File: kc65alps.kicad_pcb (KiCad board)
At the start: 2 copper layers, 304.8 x 95.3 mm, 160 parts, among them J1 Conn_01x04, J2 AVR-ISP-6, U1 ATmega32U4-AU, Y1 16MHz

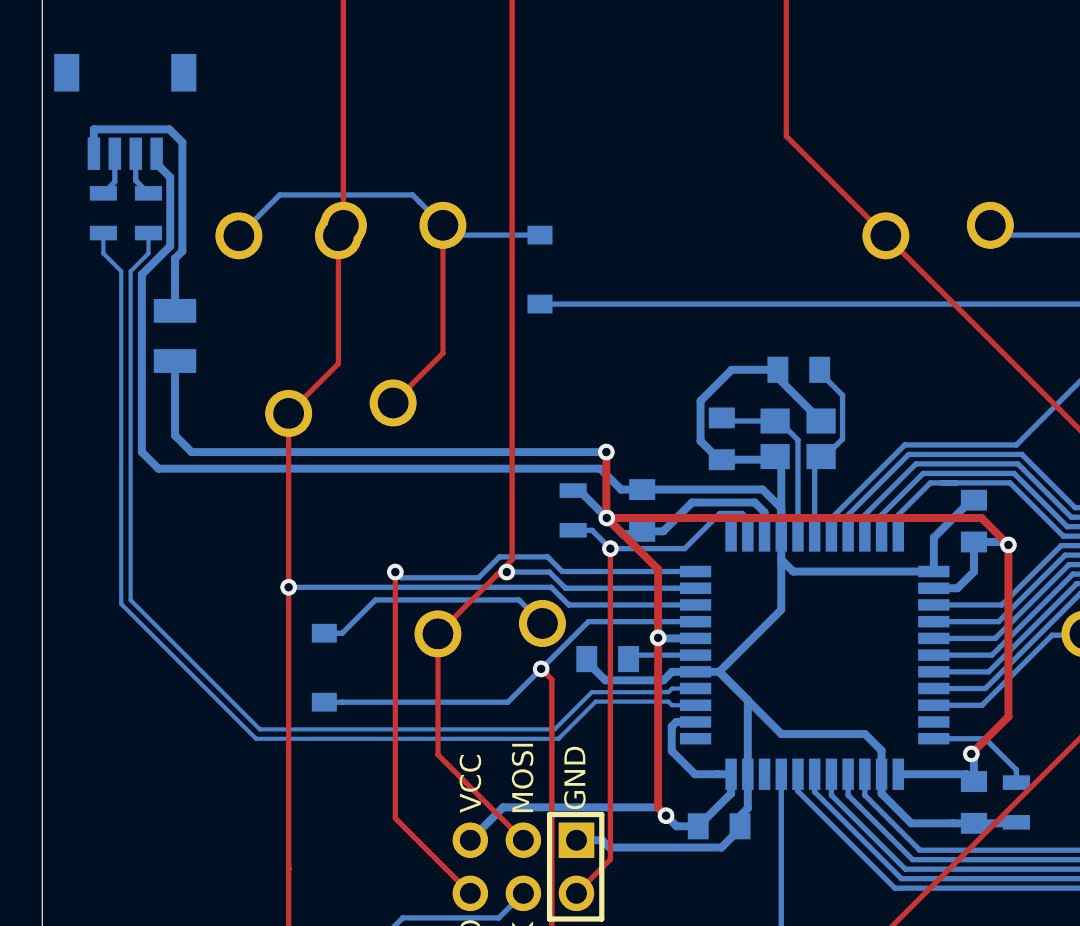
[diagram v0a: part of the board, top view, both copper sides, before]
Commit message: PCB update
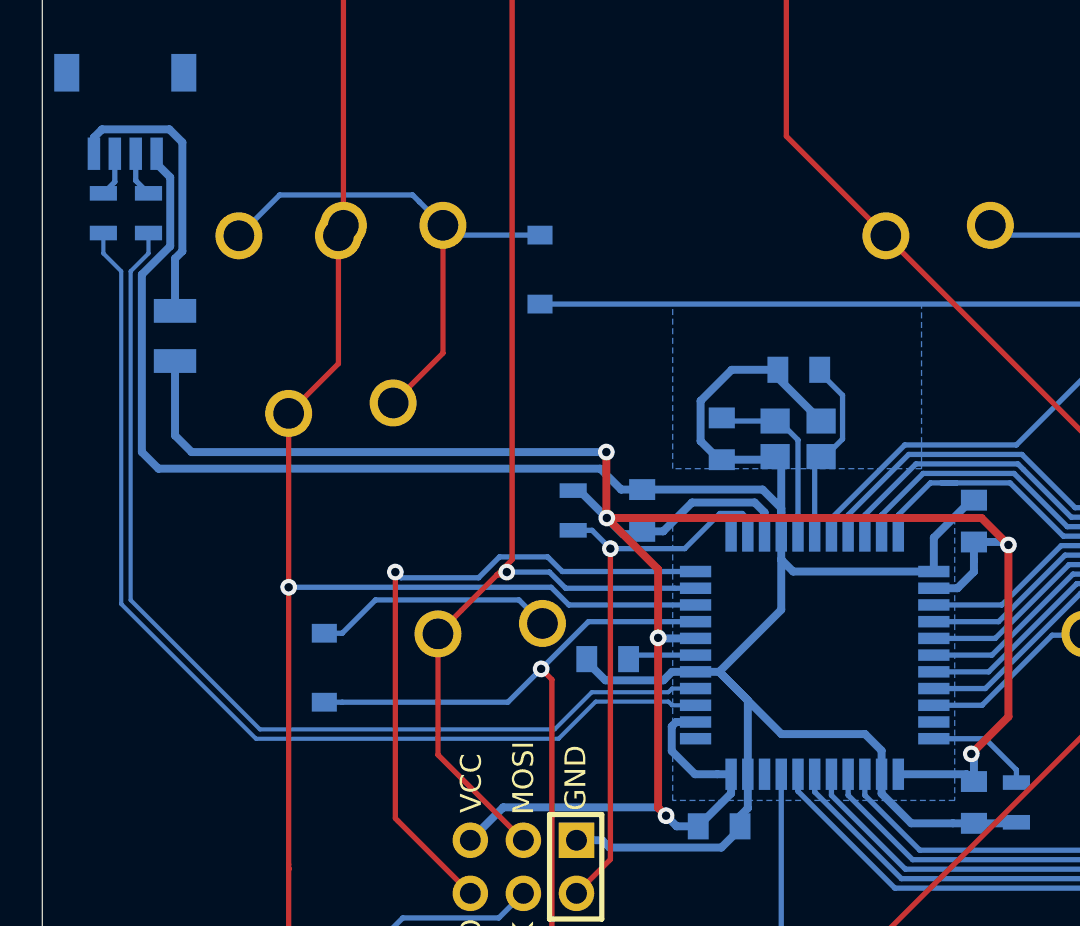
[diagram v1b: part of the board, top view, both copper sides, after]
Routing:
- added copper zone on B.Cu, net GND
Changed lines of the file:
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@@
   (segment (start 21.51875 119.075) (end 21.51875 119.55) (width 0.381) (layer B.Cu) (net 79))
   (segment (start 25.4 124.090357) (end 25.4 126.59375) (width 0.381) (layer B.Cu) (net 79))
-  (segment (start 21.51875 117.919) (end 21.528251 117.909499) (width 0.381) (layer B.Cu) (net 79))
-  (segment (start 21.51875 119.075) (end 21.51875 117.919) (width 0.381) (layer B.Cu) (net 79))
-  (segment (start 21.528251 117.909499) (end 25.131151 117.909499) (width 0.381) (layer B.Cu) (net 79))
+  (segment (start 21.51875 119.075) (end 21.51875 118.297098) (width 0.381) (layer B.Cu) (net 79))
+  (segment (start 21.906349 117.909499) (end 25.131151 117.909499) (width 0.381) (layer B.Cu) (net 79))
+  (segment (start 21.51875 118.297098) (end 21.906349 117.909499) (width 0.381) (layer B.Cu) (net 79))
   (segment (start 25.131151 117.909499) (end 25.751511 118.529859) (width 0.381) (layer B.Cu) (net 79))
   (segment (start 25.751511 118.529859) (end 25.751511 123.738846) (width 0.381) (layer B.Cu) (net 79))
@@
   (segment (start 64.1645 147.0655) (end 65.659 148.56) (width 0.254) (layer B.Cu) (net 100))
   (segment (start 61.707 147.0655) (end 64.1645 147.0655) (width 0.254) (layer B.Cu) (net 100))
+  (zone (net 2) (net_name GND) (layer B.Cu) (hatch edge 0.508)
+    (connect_pads (clearance 0.508))
+    (min_thickness 0.254)
+    (fill yes (arc_segments 32) (thermal_gap 0.508) (thermal_bridge_width 0.508))
+    (polygon
+      (pts
+        (xy 49.2125 136.525) (xy 62.70625 136.525) (xy 62.70625 150.01875) (xy 49.2125 150.01875)
+      )
+    )
+  )
+  (zone (net 2) (net_name GND) (layer B.Cu) (hatch edge 0.508)
+    (connect_pads (clearance 0.508))
+    (min_thickness 0.254)
+    (fill yes (arc_segments 32) (thermal_gap 0.508) (thermal_bridge_width 0.508))
+    (polygon
+      (pts
+        (xy 49.2125 134.14375) (xy 49.2125 126.20625) (xy 61.11875 126.20625) (xy 61.11875 134.14375)
+      )
+    )
+  )
 )
